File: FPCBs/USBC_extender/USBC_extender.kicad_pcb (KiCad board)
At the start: 2 copper layers, 16.2 x 77 mm, 2 parts, among them P1 USB_C_Mainboard, P2 USB_C_Connector

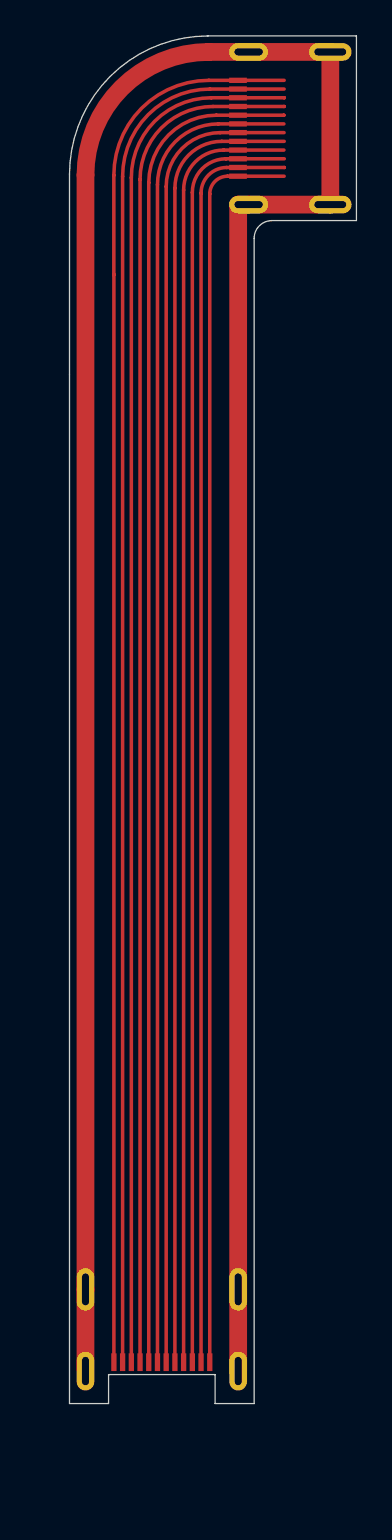
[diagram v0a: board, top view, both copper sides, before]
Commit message: Export new Gerbers and CADs
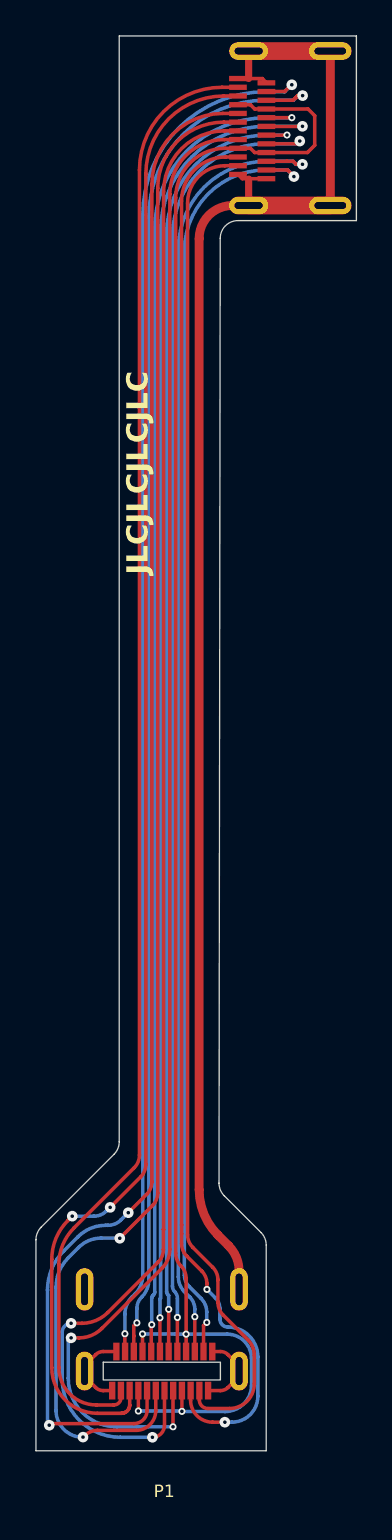
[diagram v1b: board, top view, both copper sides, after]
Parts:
- P1: footprint Leica-G9ii:FPC_Mainboard_USBC-12Pins -> Leica-G9ii:Connector_USBC-PCB-24Pins
- P2: footprint Leica-G9ii:Connector_USBC-12Pins -> Leica-G9ii:Connector_USBC-Receptacle-24Pins
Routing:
- net (no net): track 1063.0 -> 0.00 mm
- net Net-(P1-VBUS-PadA4): track 0.00 -> 99.8 mm, vias 0 -> 4
- net Net-(P1-SHIELD): track 0.00 -> 97.6 mm
- net Net-(P1-SBU2): track 0.00 -> 86.9 mm, vias 0 -> 2
- net Net-(P1-D--PadB7): track 0.00 -> 86.8 mm, vias 0 -> 2
- net Net-(P1-D+-PadB6): track 0.00 -> 85.8 mm, vias 0 -> 2
- net Net-(P1-RX1-): track 0.00 -> 84.5 mm, vias 0 -> 2
- net Net-(P1-CC2): track 0.00 -> 84.5 mm, vias 0 -> 2
- net Net-(P1-RX1+): track 0.00 -> 82.4 mm
- net Net-(P1-TX2-): track 0.00 -> 79.5 mm, vias 0 -> 2
- net Net-(P1-TX1-): track 0.00 -> 78.7 mm, vias 0 -> 2
- net Net-(P1-TX1+): track 0.00 -> 78.1 mm, vias 0 -> 2
- net Net-(P1-TX2+): track 0.00 -> 76.4 mm
- net Net-(P1-D+-PadA6): track 0.00 -> 76.3 mm, vias 0 -> 2
- net Net-(P1-CC1): track 0.00 -> 75.8 mm, vias 0 -> 2
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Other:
- board size 16.2 x 77 mm -> 18 x 79.7 mm
- board text added: "JLCJLCJLCJLC"
